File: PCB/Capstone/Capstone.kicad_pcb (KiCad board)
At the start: 2 copper layers, 81 x 48 mm, 3 parts, among them J1 ESP_Left, J2 ESP_Right, J3 TFT

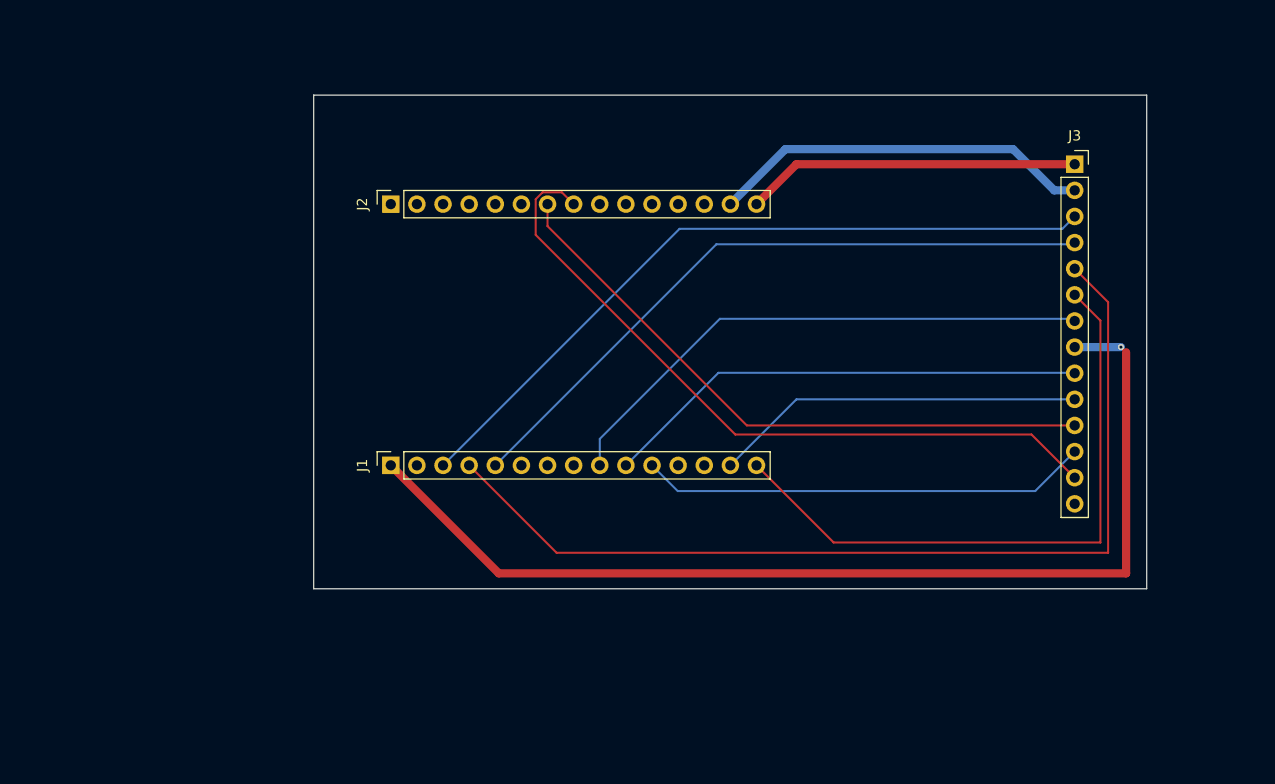
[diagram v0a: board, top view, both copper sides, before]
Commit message: Added PCB components
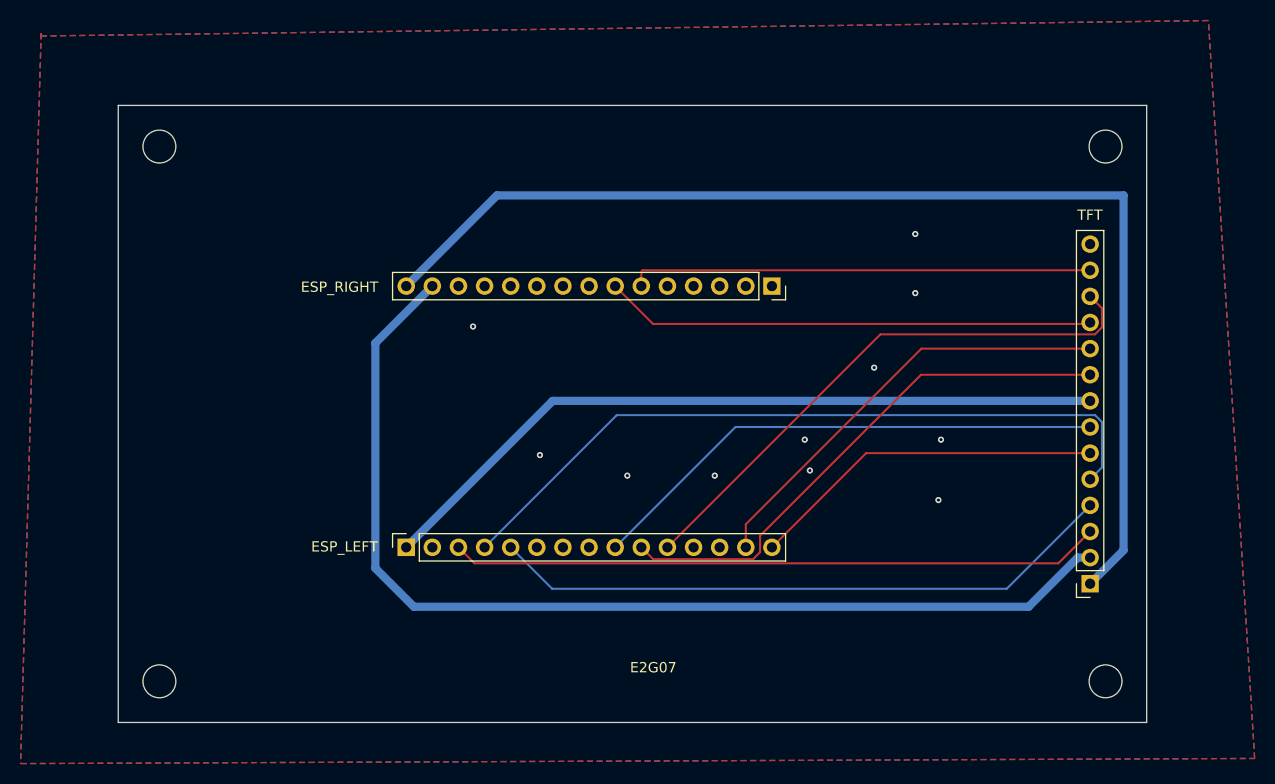
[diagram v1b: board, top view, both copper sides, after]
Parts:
- added REF**: MountingHole_3.2mm_M3, MountingHole:MountingHole_3.2mm_M3, F.Cu at (77.5, 121.0)
- added REF**: MountingHole_3.2mm_M3, MountingHole:MountingHole_3.2mm_M3, F.Cu at (169.5, 69.0)
- added REF**: MountingHole_3.2mm_M3, MountingHole:MountingHole_3.2mm_M3, F.Cu at (169.5, 121.0)
- added REF**: MountingHole_3.2mm_M3, MountingHole:MountingHole_3.2mm_M3, F.Cu at (77.5, 69.0)
- moved J3 40.8 mm to (168.0, 111.5), turned to 180 degrees
- moved J2 37.9 mm to (137.1, 82.6), turned to -90 degrees
- moved J1 8.11 mm to (101.5, 108.0)
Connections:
- J2 pad 6: unconnected-(J2-Pin_6-Pad6) -> /CTP_INT
- J2 pad 8: /CTP_INT -> unconnected-(J2-Pin_8-Pad8)
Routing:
- net /VCC: track 32.5 -> 112.5 mm
- net GND: track 37.4 -> 102.8 mm, vias 0 -> 11
- net /LED: track 102.6 -> 72.4 mm, vias 1 -> 0
- net /MOSI: track 61.7 -> 34.7 mm
- net /CTP_INT: track 70.1 -> 45.1 mm
- net /LCD_RS: track 94.6 -> 71.7 mm
- net /CTP_RST: track 61.4 -> 47.8 mm
- net /CTP_SDA: track 43.7 -> 54.6 mm
- net /LCD_CS: track 71.4 -> 63.3 mm
- net /CTP_SCL: track 36.1 -> 42.8 mm
- net /MISO: track 47.4 -> 52.5 mm
- net /LCD_RST: track 65.3 -> 61.4 mm
- net /SCK: track 53.7 -> 51.0 mm
- added copper zone on B.Cu, net GND
- added copper zone on F.Cu, net GND
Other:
- board size 81 x 48 mm -> 100 x 60 mm
- board text added: "E2G07"
- board text added: "ESP_LEFT"
- board text added: "ESP_RIGHT"
- board text added: "TFT"
